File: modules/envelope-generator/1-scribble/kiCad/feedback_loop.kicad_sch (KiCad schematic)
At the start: 7 parts, among them U1 TL074

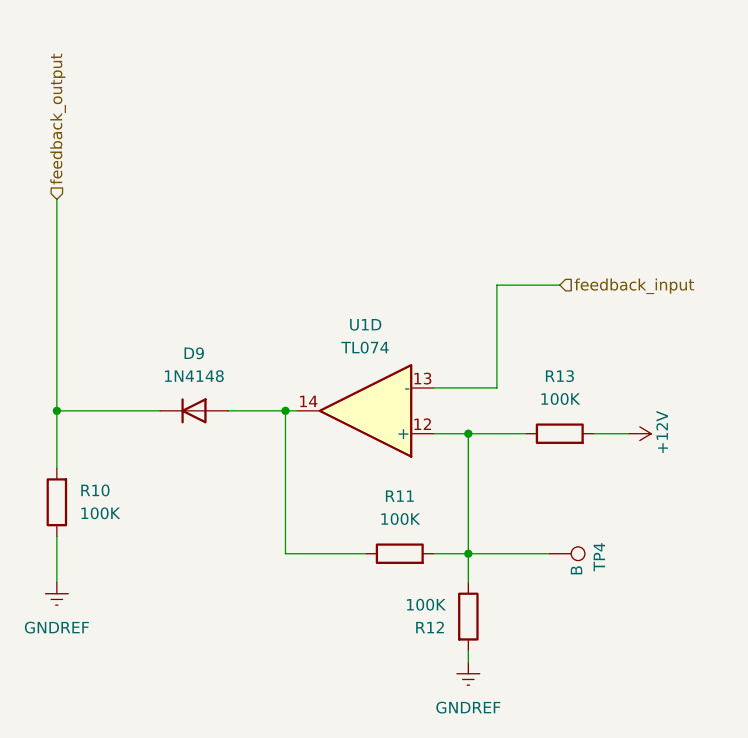
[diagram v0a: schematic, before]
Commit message: sensei models, scribble fixes
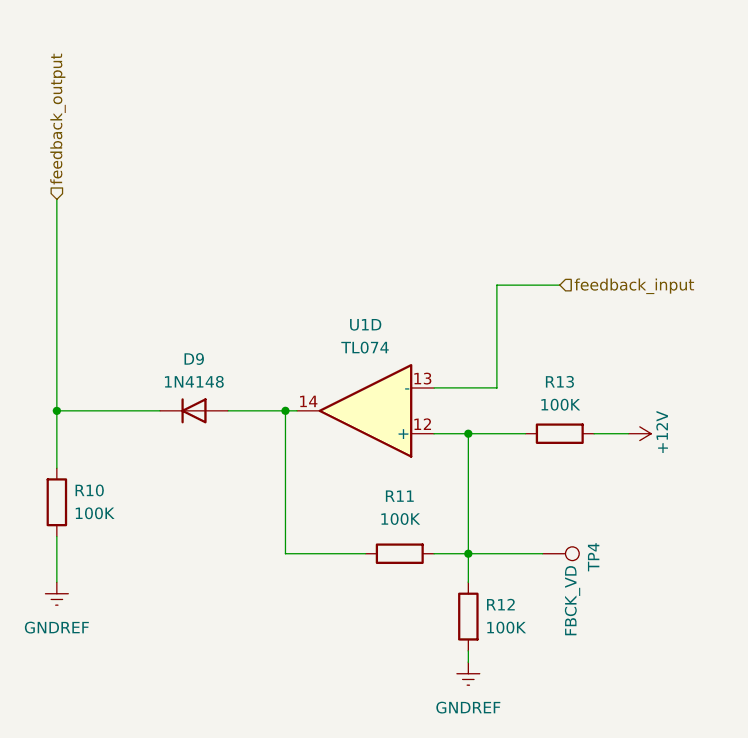
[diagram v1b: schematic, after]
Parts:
- D9: footprint synth-custom:D_default -> Synth:D_DO-35_SOD27_P7.62mm_Horizontal; symbol Diode:1N4148 -> synth:D_Signal (1N4148)
- R10, R11, R12, R13: footprint synth-custom:R_default -> Synth:R_Default (DIN0207); symbol Device:R -> synth:R_Default
- TP4: value B -> FBCK_VD
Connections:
- net +12V: now also R13.1; no longer R13.2
- net GNDREF: now also R10.2, R12.1; no longer R10.1, R12.2
- net feedback_output: now also R10.1; no longer R10.2
- net at D9.2 (A), U1.14: now also R11.2; no longer R11.1
- new net: R11.1, R12.2, R13.2, TP4.1, U1.12 (+)
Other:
- moved on the sheet: TP4

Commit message: update to BOM and add panels
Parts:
- TP4: now left out of the parts list
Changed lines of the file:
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@@
 		(unit 1)
 		(exclude_from_sim no)
-		(in_bom yes)
+		(in_bom no)
 		(on_board yes)
 		(dnp no)
